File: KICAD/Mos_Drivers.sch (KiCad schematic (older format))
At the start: 28 parts

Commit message: driver + clean clean clean
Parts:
- removed C?: 100n, symbol Device:C
- removed C?: C, symbol Device:C
- removed D? (x3): D_Schottky, symbol Device:D_Schottky
- removed D? (x4): D, symbol Device:D
- removed R? (x8): R, symbol Device:R
- removed TP? (x3): TP_POP, symbol Connector:TestPoint
- removed U?: UCC27284-Q1, Package_SO:SOIC-8_3.9x4.9mm_P1.27mm, symbol Sesame:UCC27284-Q1
- added D? (x3): SS36, Diode_SMD:D_SMA_Handsoldering, symbol Device:D_Schottky
- added R? (x4): TBD, Resistor_SMD:R_0805_2012Metric_Pad1.15x1.40mm_HandSolder, symbol Device:R
- D?: value D_Schottky -> SS36; footprint (none) -> Diode_SMD:D_SMA_Handsoldering
- gave numbers to parts that had none: 1
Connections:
- net labels added: Driver_P, Driver_S, VG_P, VG_S, VS
- net labels removed: Driver_LP, Driver_LS, Driver_RP, Driver_RS, VG_LP, VG_LS, VG_RP, VG_RS, VS_L, VS_R
- wire segments 64 -> 32
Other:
- moved on the sheet: C?, D?, TP?, U9

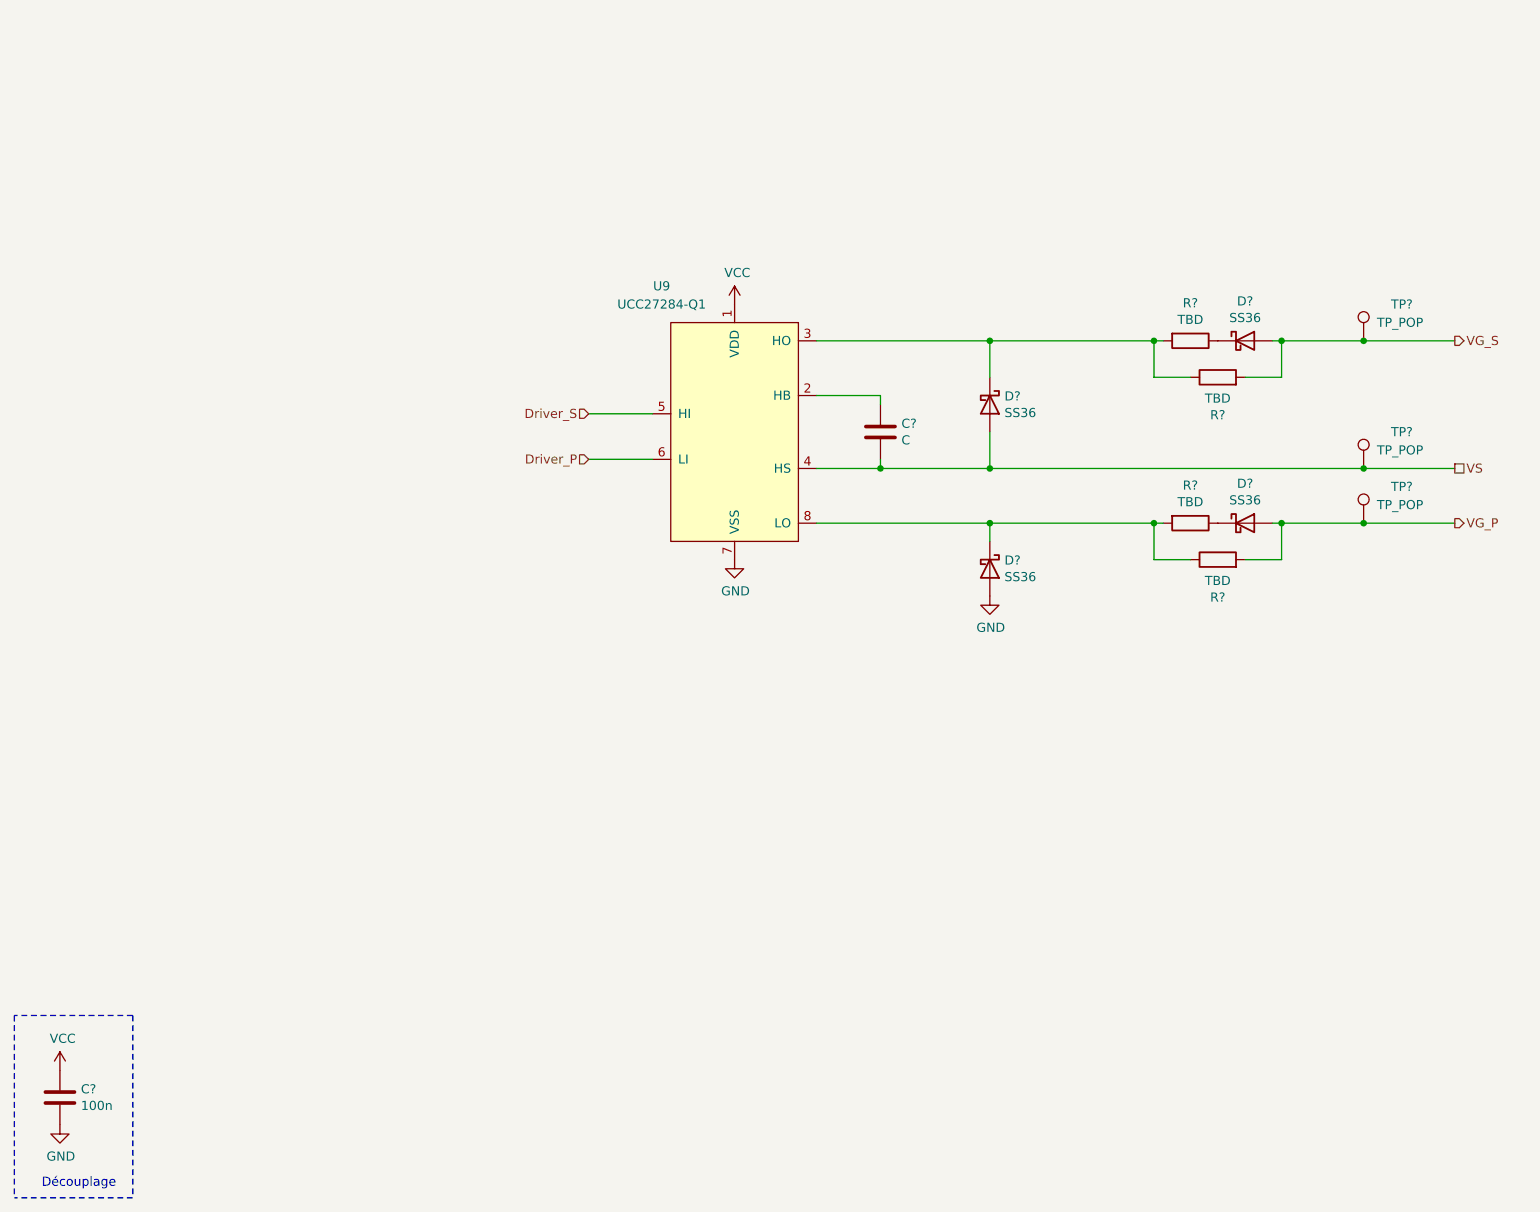
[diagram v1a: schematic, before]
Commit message: review w/ jmt
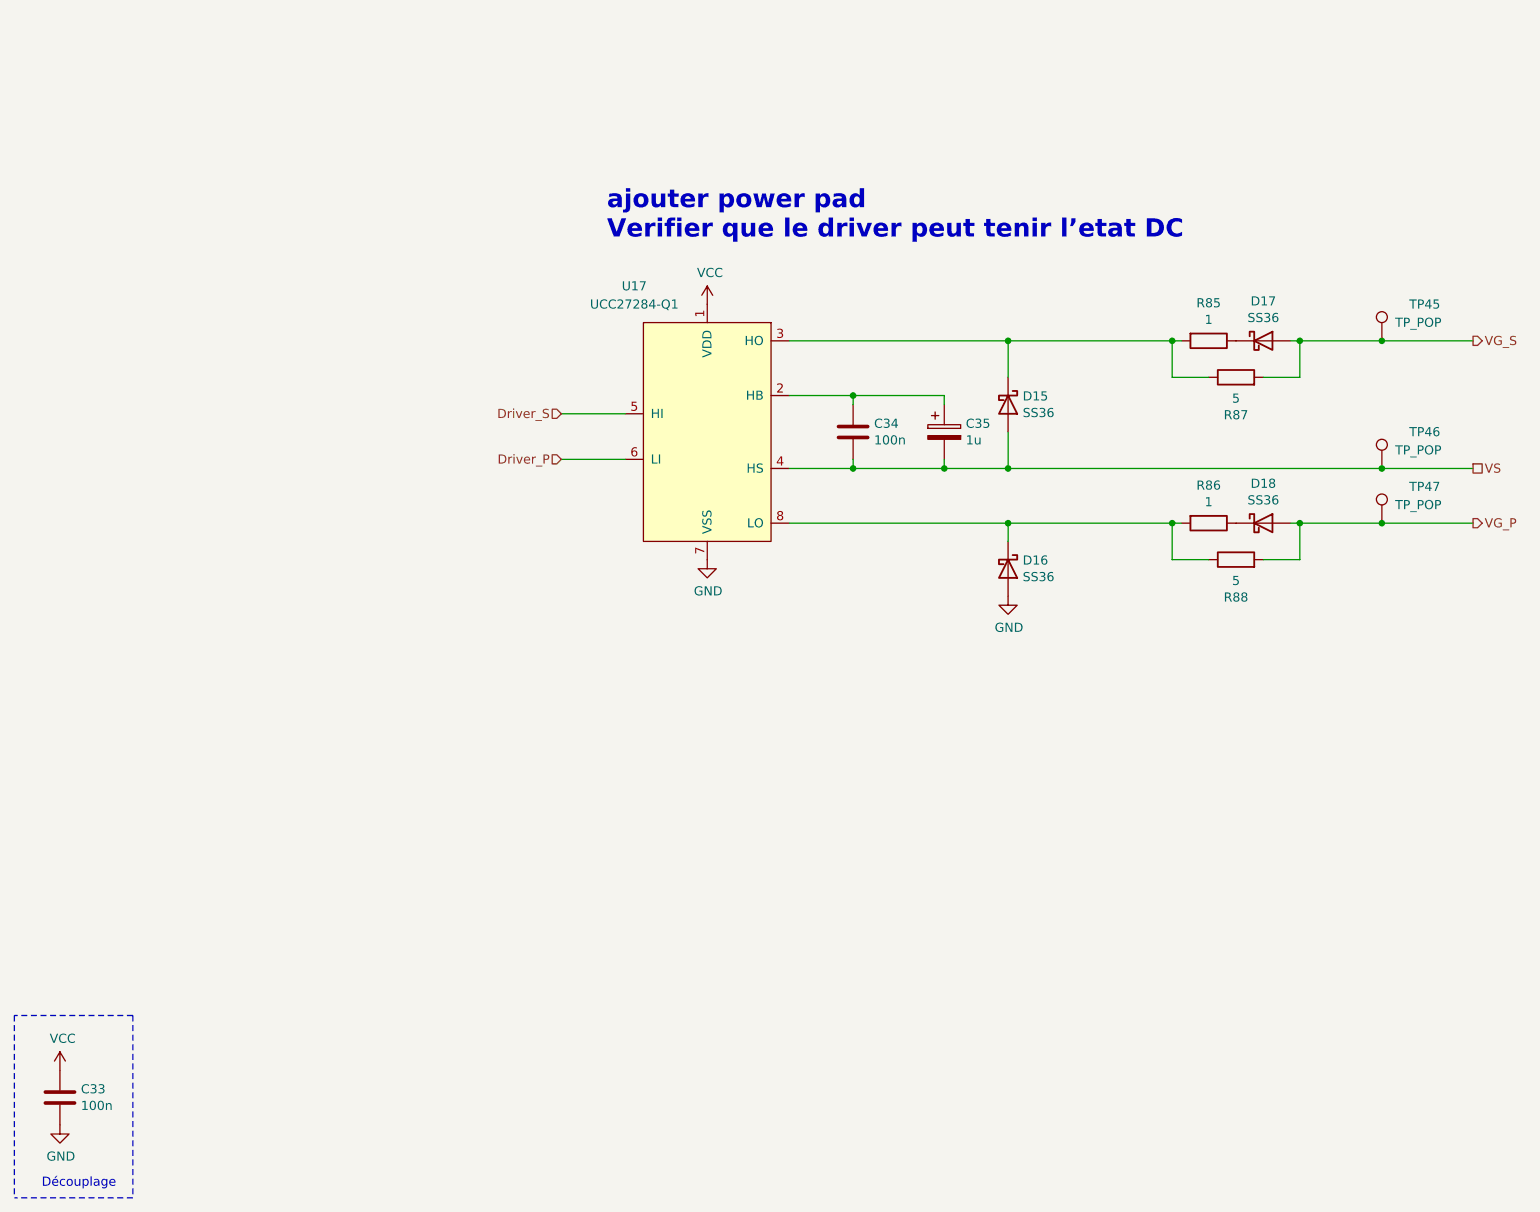
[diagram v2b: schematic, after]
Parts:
- removed C?: C, symbol Device:C
- removed D?: SS36, Diode_SMD:D_SMA_Handsoldering, symbol Device:D_Schottky
- removed R? (x2): TBD, Resistor_SMD:R_0805_2012Metric_Pad1.15x1.40mm_HandSolder, symbol Device:R
- added C24: 100n, symbol Device:C
- added C25: 1u, symbol Device:CP
- added D11: SS36, Diode_SMD:D_SMA_Handsoldering, symbol Device:D_Schottky
- added R67: 1, symbol Device:R
- added R69: 5, symbol Device:R
- R66: renamed from R?; value TBD -> 1; footprint Resistor_SMD:R_0805_2012Metric_Pad1.15x1.40mm_HandSolder -> (none)
- R68: renamed from R?; value TBD -> 5; footprint Resistor_SMD:R_0805_2012Metric_Pad1.15x1.40mm_HandSolder -> (none)
- U12: renamed from U8; footprint Package_SO:SOIC-8_3.9x4.9mm_P1.27mm -> (none)
- gave numbers to parts that had none: 7
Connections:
- net VG_P: now also D11.2 (A), R69.2
- net VS: now also C24.2, C25.2
- net at U12.2 (HB): now also C24.1, C25.1
- net at D9.1 (K), U12.8 (LO): now also R67.2, R69.1
- new net: D11.1 (K), R67.1
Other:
- note added: "ajouter power pad\nVerifier que le driver peut tenir l’etat DC"
- moved on the sheet: D15, D16, D17, R85, R87, TP45, TP46, TP47, U17
